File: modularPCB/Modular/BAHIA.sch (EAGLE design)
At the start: 3 parts

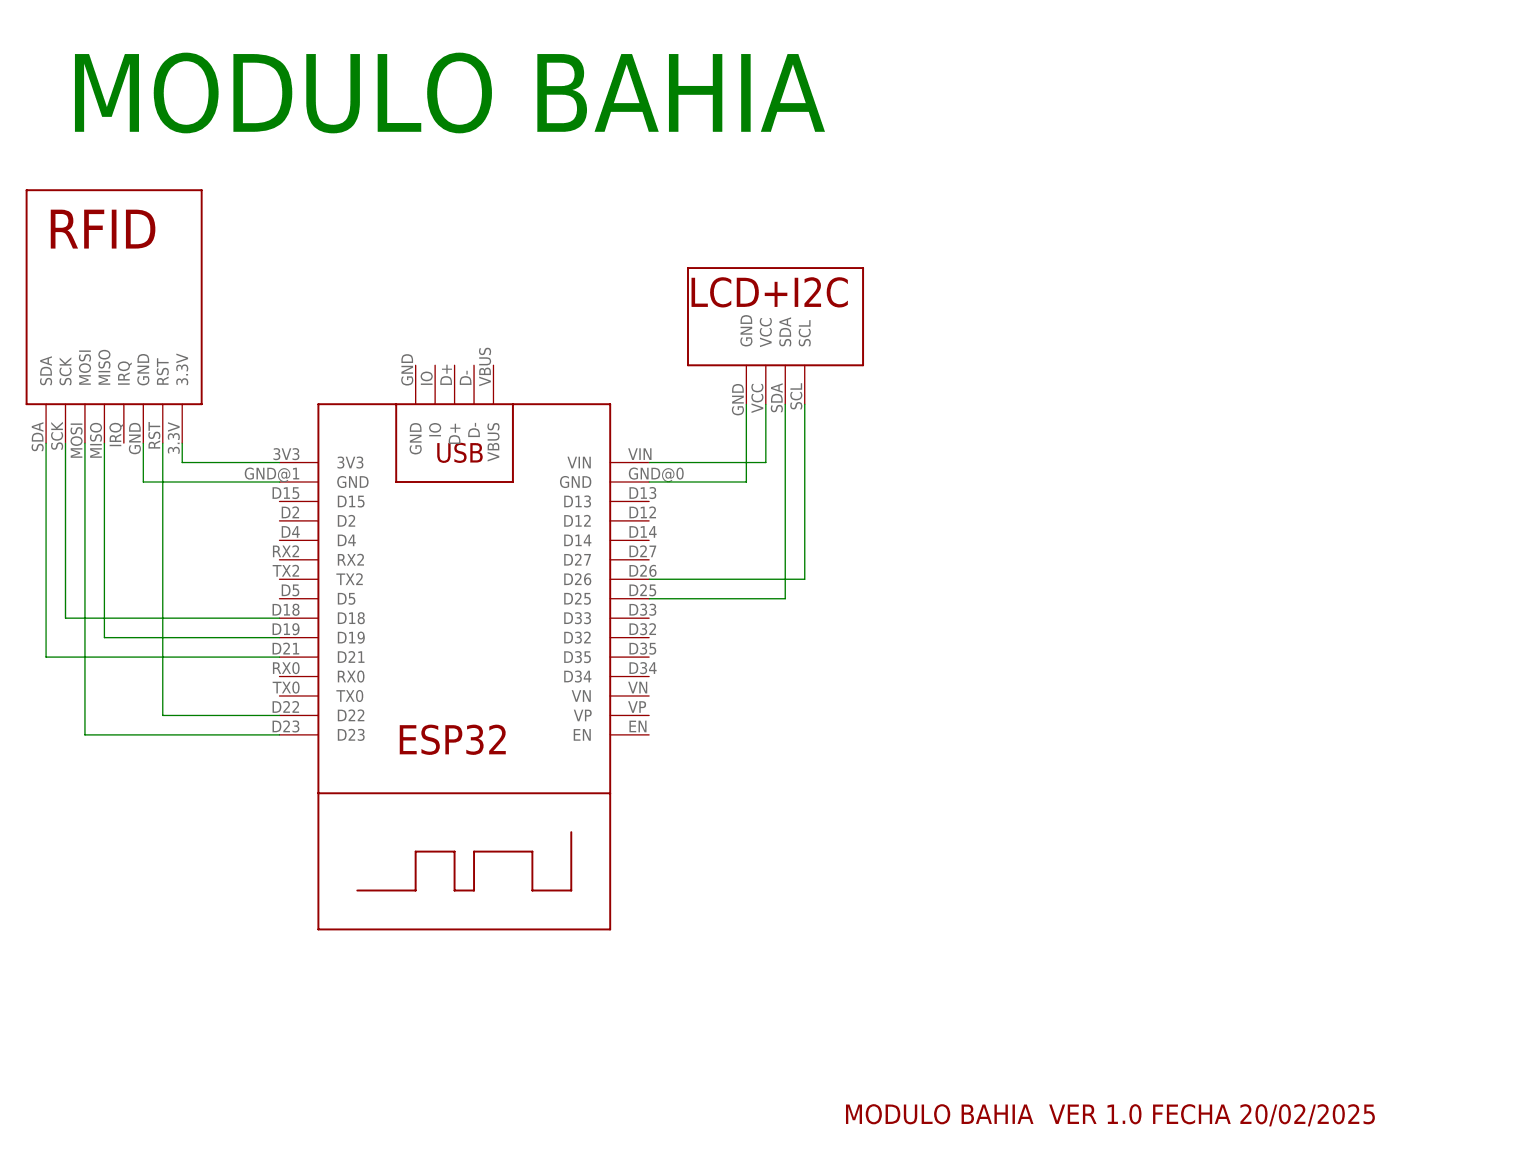
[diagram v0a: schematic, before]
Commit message: Actualización de pcbs
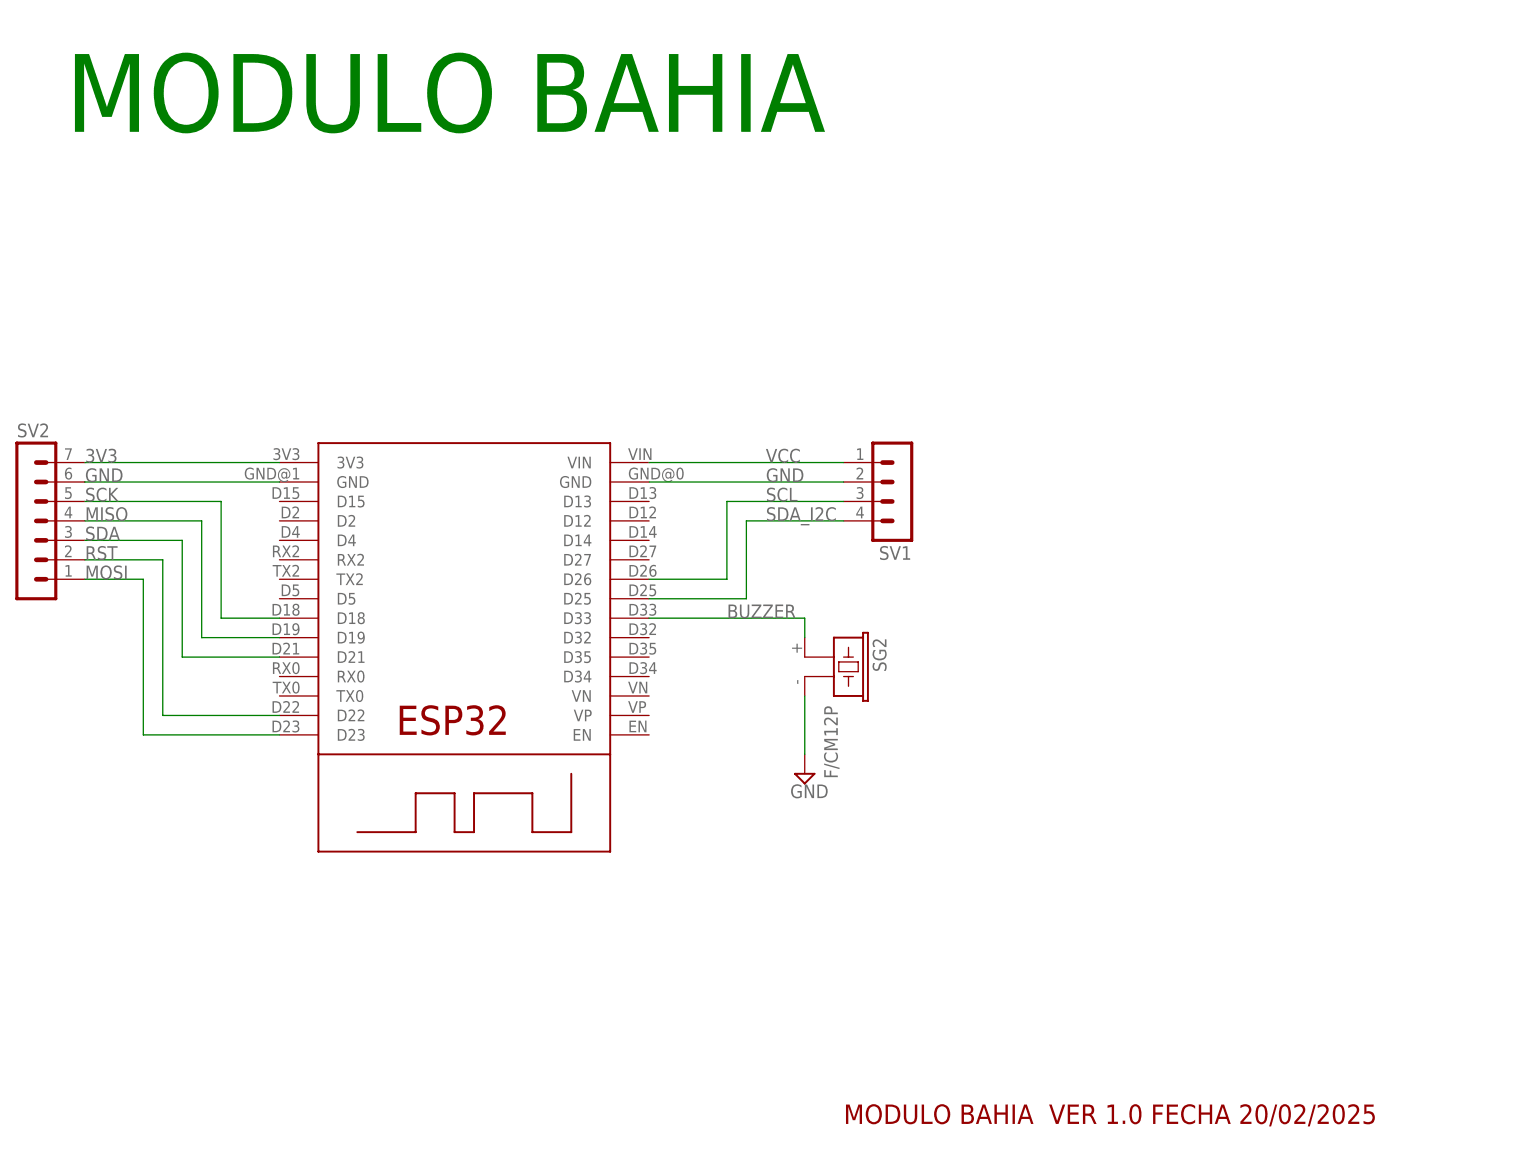
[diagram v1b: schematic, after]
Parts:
- removed U$2: LCD+I2C, MODULAR:LCD+I2C
- removed U$3: RFID, MODULAR:RFID
- added SG2: F/CM12P, buzzer:F/CM12P
- added SV1: (no value), con-lstb:MA04-1
- added SV2: (no value), con-lstb:MA07-1
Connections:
- removed net N$1: U$1.D21, U$3.SDA
- removed net N$10: U$1.D26, U$2.SCL
- removed net N$11: U$1.D25, U$2.SDA
- removed net N$2: U$1.D18, U$3.SCK
- removed net N$3: U$1.D23, U$3.MOSI
- removed net N$4: U$1.D19, U$3.MISO
- removed net N$5: U$1.GND@1, U$3.GND
- removed net N$6: U$1.D22, U$3.RST
- removed net N$7: U$1.3V3, U$3.3.3V
- removed net N$8: U$1.VIN, U$2.VCC
- removed net N$9: U$1.GND@0, U$2.GND
- new net 3V3: SV2.7, U$1.3V3
- new net BUZZER: SG2.1, U$1.D33
- new net GND: SG2.2, SV1.2, SV2.6, U$1.GND@0, U$1.GND@1
- new net MISO: SV2.4, U$1.D19
- new net MOSI: SV2.1, U$1.D23
- new net RST: SV2.2, U$1.D22
- new net SCK: SV2.5, U$1.D18
- new net SCL: SV1.3, U$1.D26
- new net SDA: SV2.3, U$1.D21
- new net SDA_I2C: SV1.4, U$1.D25
- new net VCC: SV1.1, U$1.VIN
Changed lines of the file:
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@@
 <parts>
 <part name="U$1" library="MODULAR" deviceset="ESP32WROOM" device=""/>
-<part name="U$2" library="MODULAR" deviceset="LCD+I2C" device=""/>
-<part name="U$3" library="MODULAR" deviceset="RFID" device=""/>
 <part name="FRAME2" library="frames" library_urn="urn:adsk.eagle:library:229" deviceset="A4L-LOC" device=""/>
+<part name="SV1" library="con-lstb" library_urn="urn:adsk.eagle:library:162" deviceset="MA04-1" device="" package3d_urn="urn:adsk.eagle:package:8337/1"/>
+<part name="SV2" library="con-lstb" library_urn="urn:adsk.eagle:library:162" deviceset="MA07-1" device="" package3d_urn="urn:adsk.eagle:package:8341/1"/>
+<part name="SG2" library="buzzer" library_urn="urn:adsk.eagle:library:113" deviceset="F/CM12P" device="" package3d_urn="urn:adsk.eagle:package:5265/1"/>
+<part name="SUPPLY1" library="supply2" library_urn="urn:adsk.eagle:library:372" deviceset="GND" device=""/>
 </parts>
 <sheets>
@@
 <instances>
 <instance part="U$1" gate="G$1" x="119.38" y="99.06" smashed="yes"/>
-<instance part="U$2" gate="G$1" x="160.02" y="127" smashed="yes"/>
-<instance part="U$3" gate="G$1" x="76.2" y="134.62" smashed="yes"/>
 <instance part="FRAME2" gate="G$1" x="0" y="0" smashed="yes">
 <attribute name="DRAWING_NAME" x="217.17" y="15.24" size="2.54" layer="94"/>
@@
 <attribute name="SHEET" x="230.505" y="5.08" size="2.54" layer="94"/>
 </instance>
+<instance part="SV1" gate="1" x="177.8" y="109.22" smashed="yes" rot="R180">
+<attribute name="VALUE" x="179.07" y="119.38" size="1.778" layer="96" rot="R180"/>
+<attribute name="NAME" x="179.07" y="103.378" size="1.778" layer="95" rot="R180"/>
+</instance>
+<instance part="SV2" gate="1" x="63.5" y="106.68" smashed="yes">
+<attribute name="VALUE" x="62.23" y="93.98" size="1.778" layer="96"/>
+<attribute name="NAME" x="62.23" y="117.602" size="1.778" layer="95"/>
+</instance>
+<instance part="SG2" gate="G$1" x="167.64" y="88.9" smashed="yes" rot="R270">
+<attribute name="NAME" x="173.99" y="91.44" size="1.778" layer="95" rot="R270"/>
+<attribute name="VALUE" x="167.64" y="82.55" size="1.778" layer="96" rot="R270"/>
+</instance>
+<instance part="SUPPLY1" gate="GND" x="165.1" y="73.66" smashed="yes">
+<attribute name="VALUE" x="163.195" y="70.485" size="1.778" layer="96"/>
+</instance>
 </instances>
 <busses>
 </busses>
 <nets>
-<net name="N$1" class="0">
+<net name="SDA" class="0">
 <segment>
-<pinref part="U$3" gate="G$1" pin="SDA"/>
-<wire x1="66.04" y1="116.84" x2="66.04" y2="88.9" width="0.1524" layer="91"/>
 <pinref part="U$1" gate="G$1" pin="D21"/>
-<wire x1="66.04" y1="88.9" x2="96.52" y2="88.9" width="0.1524" layer="91"/>
+<wire x1="83.82" y1="88.9" x2="96.52" y2="88.9" width="0.1524" layer="91"/>
+<pinref part="SV2" gate="1" pin="3"/>
+<wire x1="71.12" y1="104.14" x2="83.82" y2="104.14" width="0.1524" layer="91"/>
+<wire x1="83.82" y1="104.14" x2="83.82" y2="88.9" width="0.1524" layer="91"/>
+<label x="71.12" y="104.14" size="1.778" layer="95"/>
 </segment>
 </net>
-<net name="N$2" class="0">
+<net name="SCK" class="0">
 <segment>
-<pinref part="U$3" gate="G$1" pin="SCK"/>
 <pinref part="U$1" gate="G$1" pin="D18"/>
-<wire x1="68.58" y1="116.84" x2="68.58" y2="93.98" width="0.1524" layer="91"/>
-<wire x1="68.58" y1="93.98" x2="96.52" y2="93.98" width="0.1524" layer="91"/>
+<wire x1="88.9" y1="93.98" x2="96.52" y2="93.98" width="0.1524" layer="91"/>
+<pinref part="SV2" gate="1" pin="5"/>
+<wire x1="71.12" y1="109.22" x2="88.9" y2="109.22" width="0.1524" layer="91"/>
+<wire x1="88.9" y1="109.22" x2="88.9" y2="93.98" width="0.1524" layer="91"/>
+<label x="71.12" y="109.22" size="1.778" layer="95"/>
 </segment>
 </net>
-<net name="N$3" class="0">
+<net name="MOSI" class="0">
 <segment>
-<pinref part="U$3" gate="G$1" pin="MOSI"/>
-<wire x1="71.12" y1="116.84" x2="71.12" y2="78.74" width="0.1524" layer="91"/>
 <pinref part="U$1" gate="G$1" pin="D23"/>
-<wire x1="71.12" y1="78.74" x2="96.52" y2="78.74" width="0.1524" layer="91"/>
+<wire x1="78.74" y1="78.74" x2="96.52" y2="78.74" width="0.1524" layer="91"/>
+<pinref part="SV2" gate="1" pin="1"/>
+<wire x1="71.12" y1="99.06" x2="78.74" y2="99.06" width="0.1524" layer="91"/>
+<wire x1="78.74" y1="99.06" x2="78.74" y2="78.74" width="0.1524" layer="91"/>
+<label x="71.12" y="99.06" size="1.778" layer="95"/>
 </segment>
 </net>
-<net name="N$4" class="0">
+<net name="MISO" class="0">
 <segment>
-<pinref part="U$3" gate="G$1" pin="MISO"/>
 <pinref part="U$1" gate="G$1" pin="D19"/>
-<wire x1="73.66" y1="116.84" x2="73.66" y2="91.44" width="0.1524" layer="91"/>
-<wire x1="73.66" y1="91.44" x2="96.52" y2="91.44" width="0.1524" layer="91"/>
+<wire x1="86.36" y1="91.44" x2="96.52" y2="91.44" width="0.1524" layer="91"/>
+<pinref part="SV2" gate="1" pin="4"/>
+<wire x1="71.12" y1="106.68" x2="86.36" y2="106.68" width="0.1524" layer="91"/>
+<wire x1="86.36" y1="106.68" x2="86.36" y2="91.44" width="0.1524" layer="91"/>
+<label x="71.12" y="106.68" size="1.778" layer="95"/>
 </segment>
 </net>
-<net name="N$5" class="0">
+<net name="GND" class="0">
 <segment>
-<pinref part="U$3" gate="G$1" pin="GND"/>
 <pinref part="U$1" gate="G$1" pin="GND@1"/>
-<wire x1="78.74" y1="116.84" x2="78.74" y2="111.76" width="0.1524" layer="91"/>
-<wire x1="78.74" y1="111.76" x2="96.52" y2="111.76" width="0.1524" layer="91"/>
+<pinref part="SV2" gate="1" pin="6"/>
+<wire x1="71.12" y1="111.76" x2="96.52" y2="111.76" width="0.1524" layer="91"/>
+<label x="71.12" y="111.76" size="1.778" layer="95"/>
+</segment>
+<segment>
+<pinref part="U$1" gate="G$1" pin="GND@0"/>
+<pinref part="SV1" gate="1" pin="2"/>
+<wire x1="144.78" y1="111.76" x2="170.18" y2="111.76" width="0.1524" layer="91"/>
+<label x="160.02" y="111.76" size="1.778" layer="95"/>
+</segment>
+<segment>
+<pinref part="SG2" gate="G$1" pin="2"/>
+<pinref part="SUPPLY1" gate="GND" pin="GND"/>
+<wire x1="165.1" y1="83.82" x2="165.1" y2="76.2" width="0.1524" layer="91"/>
 </segment>
 </net>
-<net name="N$6" class="0">
+<net name="RST" class="0">
 <segment>
-<pinref part="U$3" gate="G$1" pin="RST"/>
 <pinref part="U$1" gate="G$1" pin="D22"/>
-<wire x1="81.28" y1="116.84" x2="81.28" y2="81.28" width="0.1524" layer="91"/>
+<pinref part="SV2" gate="1" pin="2"/>
+<wire x1="71.12" y1="101.6" x2="81.28" y2="101.6" width="0.1524" layer="91"/>
+<wire x1="81.28" y1="101.6" x2="81.28" y2="81.28" width="0.1524" layer="91"/>
 <wire x1="81.28" y1="81.28" x2="96.52" y2="81.28" width="0.1524" layer="91"/>
+<label x="71.12" y="101.6" size="1.778" layer="95"/>
 </segment>
 </net>
-<net name="N$7" class="0">
+<net name="3V3" class="0">
 <segment>
-<pinref part="U$3" gate="G$1" pin="3.3V"/>
 <pinref part="U$1" gate="G$1" pin="3V3"/>
-<wire x1="83.82" y1="116.84" x2="83.82" y2="114.3" width="0.1524" layer="91"/>
-<wire x1="83.82" y1="114.3" x2="96.52" y2="114.3" width="0.1524" layer="91"/>
+<wire x1="71.12" y1="114.3" x2="96.52" y2="114.3" width="0.1524" layer="91"/>
+<pinref part="SV2" gate="1" pin="7"/>
+<label x="71.12" y="114.3" size="1.778" layer="95"/>
 </segment>
 </net>
-<net name="N$8" class="0">
+<net name="VCC" class="0">
 <segment>
 <pinref part="U$1" gate="G$1" pin="VIN"/>
-<wire x1="144.78" y1="114.3" x2="160.02" y2="114.3" width="0.1524" layer="91"/>
-<pinref part="U$2" gate="G$1" pin="VCC"/>
-<wire x1="160.02" y1="114.3" x2="160.02" y2="121.92" width="0.1524" layer="91"/>
+<pinref part="SV1" gate="1" pin="1"/>
+<wire x1="144.78" y1="114.3" x2="170.18" y2="114.3" width="0.1524" layer="91"/>
+<label x="160.02" y="114.3" size="1.778" layer="95"/>
 </segment>
 </net>
-<net name="N$9" class="0">
+<net name="SCL" class="0">
 <segment>
-<pinref part="U$1" gate="G$1" pin="GND@0"/>
-<pinref part="U$2" gate="G$1" pin="GND"/>
-<wire x1="144.78" y1="111.76" x2="157.48" y2="111.76" width="0.1524" layer="91"/>
-<wire x1="157.48" y1="111.76" x2="157.48" y2="121.92" width="0.1524" layer="91"/>
+<pinref part="U$1" gate="G$1" pin="D26"/>
+<wire x1="154.94" y1="99.06" x2="144.78" y2="99.06" width="0.1524" layer="91"/>
+<pinref part="SV1" gate="1" pin="3"/>
+<wire x1="154.94" y1="99.06" x2="154.94" y2="109.22" width="0.1524" layer="91"/>
+<wire x1="154.94" y1="109.22" x2="170.18" y2="109.22" width="0.1524" layer="91"/>
+<label x="160.02" y="109.22" size="1.778" layer="95"/>
 </segment>
 </net>
-<net name="N$10" class="0">
+<net name="SDA_I2C" class="0">
 <segment>
-<pinref part="U$2" gate="G$1" pin="SCL"/>
-<pinref part="U$1" gate="G$1" pin="D26"/>
-<wire x1="165.1" y1="121.92" x2="165.1" y2="99.06" width="0.1524" layer="91"/>
-<wire x1="165.1" y1="99.06" x2="144.78" y2="99.06" width="0.1524" layer="91"/>
+<pinref part="U$1" gate="G$1" pin="D25"/>
+<wire x1="144.78" y1="96.52" x2="157.48" y2="96.52" width="0.1524" layer="91"/>
+<pinref part="SV1" gate="1" pin="4"/>
+<wire x1="157.48" y1="96.52" x2="157.48" y2="106.68" width="0.1524" layer="91"/>
+<wire x1="157.48" y1="106.68" x2="170.18" y2="106.68" width="0.1524" layer="91"/>
+<label x="160.02" y="106.68" size="1.778" layer="95"/>
 </segment>
 </net>
-<net name="N$11" class="0">
+<net name="BUZZER" class="0">
 <segment>
-<pinref part="U$1" gate="G$1" pin="D25"/>
-<pinref part="U$2" gate="G$1" pin="SDA"/>
-<wire x1="144.78" y1="96.52" x2="162.56" y2="96.52" width="0.1524" layer="91"/>
-<wire x1="162.56" y1="96.52" x2="162.56" y2="121.92" width="0.1524" layer="91"/>
+<pinref part="U$1" gate="G$1" pin="D33"/>
+<pinref part="SG2" gate="G$1" pin="1"/>
+<wire x1="144.78" y1="93.98" x2="165.1" y2="93.98" width="0.1524" layer="91"/>
+<wire x1="165.1" y1="93.98" x2="165.1" y2="91.44" width="0.1524" layer="91"/>
+<label x="154.94" y="93.98" size="1.778" layer="95"/>
 </segment>
 </net>
@@
 will not be understood (or retained) with this version.
 </note>
+<note version="8.3" severity="warning">
+Since Version 8.3, EAGLE supports the association of 3D packages
+with devices in libraries, schematics, and board files. Those 3D
+packages will not be understood (or retained) with this version.
+</note>
 </compatibility>
